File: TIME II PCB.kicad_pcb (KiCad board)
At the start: 2 copper layers, 89.9 x 62.7 mm, 116 parts, among them J1 USB_C_Receptacle, J2 SD_Card, J21 Conn_01x02_Male, J3 Conn_01x02_Male, J4 Conn_01x06_Pin, J5 Conn_01x06_Pin, J6 Conn_01x06_Pin, J7 Conn_01x06_Pin, J8 Conn_01x06_Pin, Q1 VNP10N07, Q2 VNP10N07, Q3 VNP10N07, Q4 VNP10N07, Q5 VNP10N07, Q6 NMOS, Q7 PMOS, SW1 PTS647SM38SMTR2LFS, SW2 PTS647SM38SMTR2LFS, SW3 SW_SPDT, SW4 SW_SPDT, SW5 SW_SPDT, SW6 SW_SPDT, SW7 SW_SPDT, U1 ESP32-S2-SOLO, U2 ADP2303, U3 LTC4420CMSE-PBF

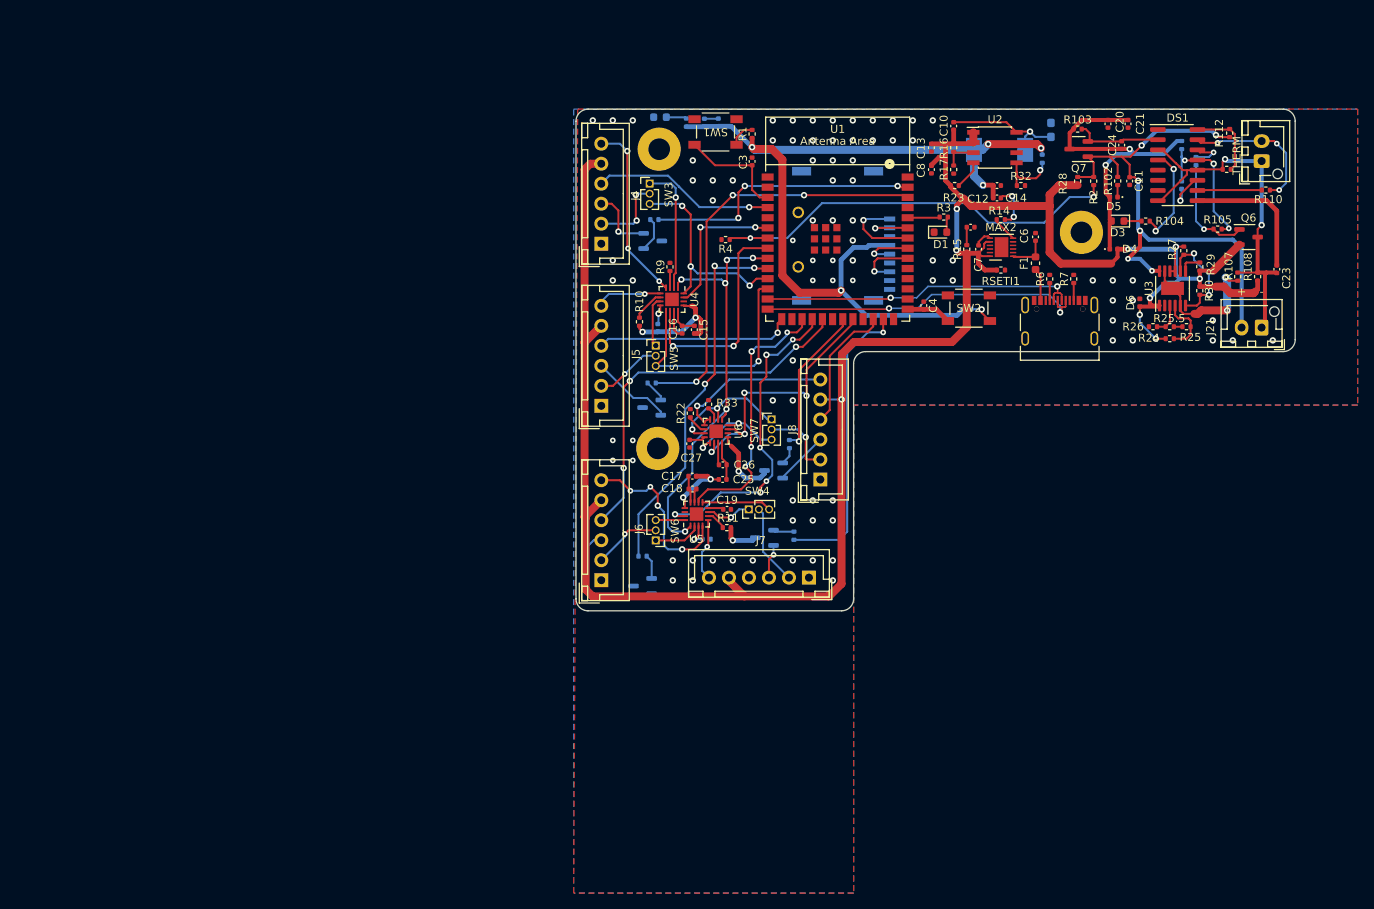
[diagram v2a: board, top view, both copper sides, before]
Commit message: new board
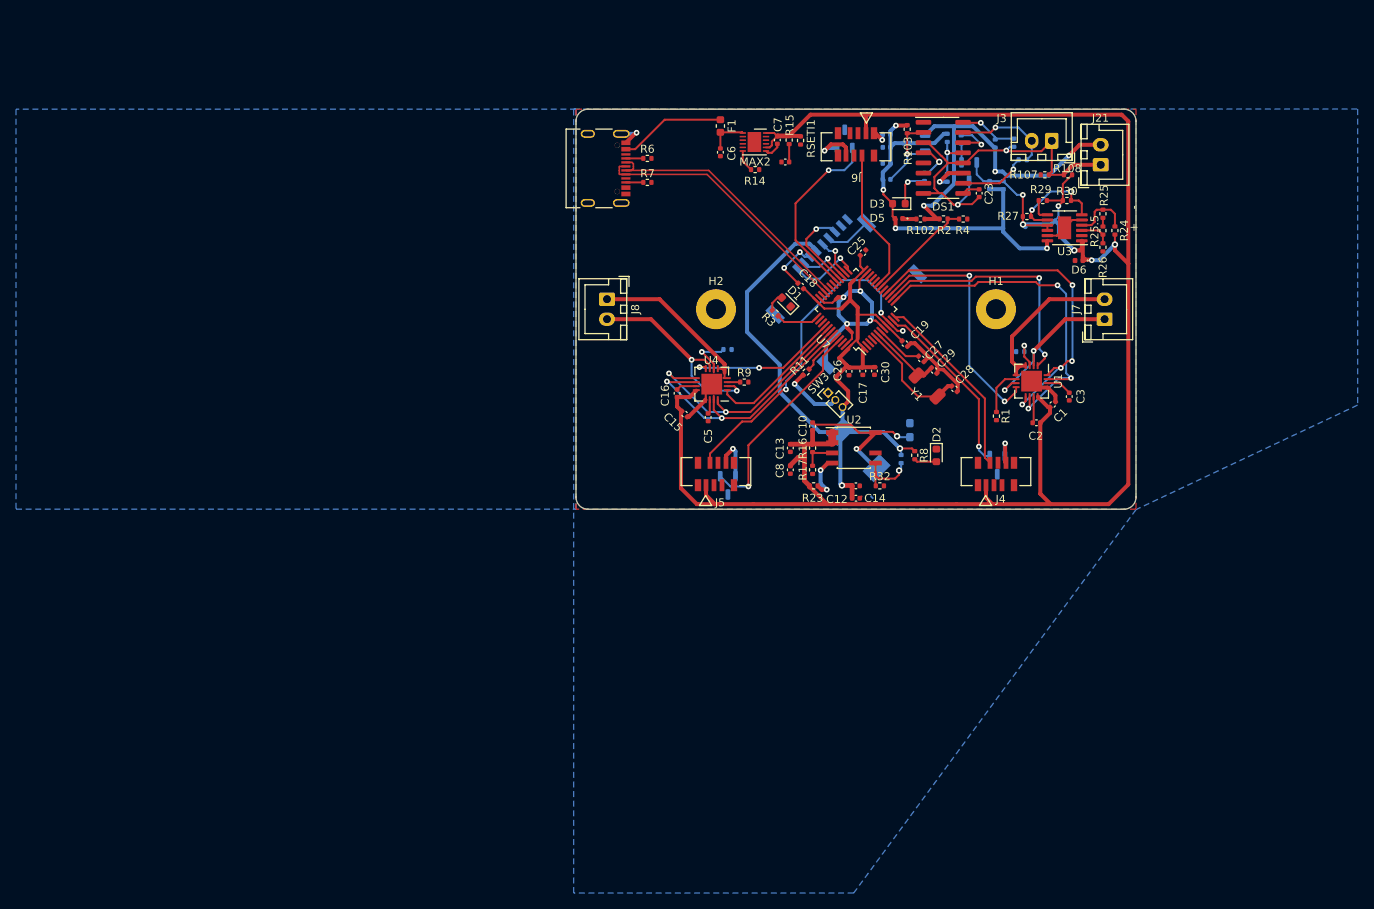
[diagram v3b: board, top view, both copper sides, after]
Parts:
- removed ? (x2): , 
- removed C4: .1uF, Capacitor_SMD:C_0402_1005Metric
- removed Q2, Q3: VNP10N07, Package_TO_SOT_SMD:SOT-23-3
- removed R105: R, Resistor_SMD:R_0402_1005Metric
- removed R13, R18, R19, R21, R5: 1.5k, Resistor_SMD:R_0402_1005Metric
- removed R20: 10k, Resistor_SMD:R_0402_1005Metric
- removed R22, R33: .33, Resistor_SMD:R_0402_1005Metric
- removed REF**: MountingHole_2.7mm_M2.5_Pad, MountingHole:MountingHole_2.7mm_M2.5_Pad
- removed SW1, SW2: PTS647SM38SMTR2LFS, button:SW_PTS647SM38SMTR2LFS_CNK
- removed SW4, SW5, SW6, SW7: SW_SPDT, Connector_PinHeader_1.27mm:PinHeader_1x03_P1.27mm_Vertical
- removed U5, U6: ~, Package_DFN_QFN:QFN-16-1EP_3x3mm_P0.5mm_EP1.7x1.7mm
- added C28: 26pF, Capacitor_SMD:C_0402_1005Metric, F.Cu at (187.7, 98.6)
- added C29: 26pF, Capacitor_SMD:C_0402_1005Metric, F.Cu at (185.2, 96.3)
- added C30: 100nF, Capacitor_SMD:C_0402_1005Metric, F.Cu at (177.7, 96.3)
- added H1: MountingHole_Pad, MountingHole:MountingHole_2.5mm_Pad, F.Cu at (192.9, 88.6)
- added H2: MountingHole_Pad, MountingHole:MountingHole_2.5mm_Pad, F.Cu at (157.9, 88.6)
- added U7: STM32F103C8Tx, Package_QFP:LQFP-48_7x7mm_P0.5mm, F.Cu at (175.4, 88.6)
- added Y1: 16 khz, crystal:abm3, F.Cu at (184.3, 98.2)
- C1: value 1uF -> 10uF; moved to F.Cu
- C11, C20, C21, C24, D4, Q6, Q7, R10, R104, R110, R112, R113, R28: moved to B.Cu
- C17, C25: value 10uF -> 100nF
- C18: value 0.01uF -> 100nF
- C19, C27: value 2.2pF -> 100nF
- C2: value .1uF -> 0.01uF; moved to F.Cu
- C26: value 0.01uF -> 10uF
- C3: value .1uF -> 2.2pF
- C5, D2, R8: moved to F.Cu
- J21, J3: footprint Connector_JST:JST_XH_B2B-XH-AM_1x02_P2.50mm_Vertical -> Connector_JST:JST_XH_B2B-XH-A_1x02_P2.50mm_Vertical
- J4, J5, J6: value Conn_01x06_Pin -> Conn_01x06; footprint Connectors_JST:JST_XH_B06B-XH-A_06x2.50mm_Straight -> ffc_conn:CON_525590652_MOL
- J7, J8: value Conn_01x06_Pin -> Conn_01x02_Male; footprint Connectors_JST:JST_XH_B06B-XH-A_06x2.50mm_Straight -> Connector_JST:JST_XH_B2B-XH-A_1x02_P2.50mm_Vertical
- R1: value 10k -> .33
- R11: value .33 -> 10k
- U1: value ESP32-S2-SOLO -> ~; footprint Espressif:ESP32-S2-SOLO -> Package_DFN_QFN:WQFN-16-1EP_4x4mm_P0.5mm_EP2.6x2.6mm
- U4: footprint Package_DFN_QFN:QFN-16-1EP_3x3mm_P0.5mm_EP1.7x1.7mm -> Package_DFN_QFN:WQFN-16-1EP_4x4mm_P0.5mm_EP2.6x2.6mm
- moved J6 63.1 mm to (175.4, 68.0), turned to 180 degrees
- moved Q5 61.3 mm to (174.0, 67.3), turned to 90 degrees
- moved J1 61.1 mm to (143.2, 71.0), turned to -90 degrees
- moved J4 57.1 mm to (192.9, 109.2), turned to 0 degrees
- moved C2 56.0 mm to (198.0, 102.8), turned to 180 degrees
- moved C1 54.7 mm to (200.0, 100.5), turned to 45 degrees
- moved R7 54.6 mm to (149.3, 72.7), turned to 0 degrees
- moved D2 54.6 mm to (185.4, 106.9), turned to -90 degrees
- moved R6 52.5 mm to (149.3, 69.8), turned to 0 degrees
- moved Q4 51.4 mm to (193.1, 108.1), turned to -90 degrees
- moved R8 50.4 mm to (182.7, 106.9), turned to -90 degrees
- moved C3 49.4 mm to (202.1, 99.5)
- moved J7 49.1 mm to (206.5, 89.8), turned to 90 degrees
- moved R1 46.6 mm to (193.0, 102.0), turned to -90 degrees
- moved R12 45.7 mm to (195.9, 93.9), turned to 180 degrees
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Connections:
- C1 pad 1: 3v3 -> 5v
- C15 pad 1: Net-(U4-VM) -> 5v
- C16 pad 1: Net-(U4-VM) -> 5v
- C17 pad 1: Net-(U5-VM) -> 3v3
- C18 pad 1: Net-(U5-VM) -> 3v3
- C18 pad 2: Net-(U5-VCP) -> GND
- C19 pad 1: Net-(U5-NFAULT) -> 3v3
- C2 pad 1: 3v3 -> 5v
- C2 pad 2: GND -> Net-(U1-VCP)
- C20 pad 1: LOAD -> BAT
- C21 pad 1: LOAD -> BAT
- C24 pad 1: LOAD -> BAT
- C25 pad 1: Net-(U6-VM) -> 3v3
- C26 pad 1: Net-(U6-VM) -> 3v3
- C26 pad 2: Net-(U6-VCP) -> GND
- C27 pad 1: Net-(U6-NFAULT) -> /nrst
- C3 pad 1: GND -> Net-(U1-VINT)
- C3 pad 2: Net-(U1-EN) -> GND
- C5 pad 1: Net-(U4-NFAULT) -> Net-(U4-VINT)
- D3 pad 2: LOAD -> BAT
- D4 pad 1: LOAD -> BAT
- D5 pad 2: LOAD -> BAT
- J21 pad 2: BAT -> BAT_REAL
- J4 pad 1: GND -> 5v
- J4 pad 2: ACTUATOR_1 -> therm_1
- J4 pad 3: Net-(J4-Pin_3) -> unconnected-(J4-Pin_3-Pad3)
- J4 pad 4: therm_1 -> GND
- J4 pad 5: 5v -> unconnected-(J4-Pin_5-Pad5)
- J4 pad 6: MOTOR_1A -> Net-(J4-Pin_6)
- J5 pad 1: GND -> 5v
- J5 pad 2: ACTUATOR_2 -> therm_2
- J5 pad 3: Net-(J5-Pin_3) -> unconnected-(J5-Pin_3-Pad3)
- J5 pad 4: therm_2 -> GND
- J5 pad 5: 5v -> unconnected-(J5-Pin_5-Pad5)
- J5 pad 6: MOTOR_2A -> Net-(J5-Pin_6)
- J6 pad 1: GND -> 5v
- J6 pad 2: ACTUATOR_3 -> therm_3
- J6 pad 3: Net-(J6-Pin_3) -> unconnected-(J6-Pin_3-Pad3)
- J6 pad 4: therm_3 -> GND
- J6 pad 5: 5v -> unconnected-(J6-Pin_5-Pad5)
- J6 pad 6: MOTOR_3A -> Net-(J6-Pin_6)
- J7 pad 1: GND -> MOTOR_2
- J7 pad 2: ACTUATOR_4 -> MOTOR_2A
- J8 pad 1: GND -> MOTOR_1A
- J8 pad 2: ACTUATOR_5 -> MOTOR_1
- Q1 pad 1: Net-(Q1-G) -> heater_2
- Q1 pad 2: Net-(J5-Pin_3) -> Net-(J5-Pin_6)
- Q4 pad 1: Net-(Q4-G) -> heater_1
- Q4 pad 2: Net-(J4-Pin_3) -> Net-(J4-Pin_6)
- Q5 pad 1: Net-(Q5-G) -> heater_3
- Q5 pad 2: Net-(J6-Pin_3) -> Net-(J6-Pin_6)
- Q7 pad 1: BAT -> BAT_REAL
- Q7 pad 3: LOAD -> BAT
- R1 pad 1: 3v3 -> Net-(U1-BISEN)
- R1 pad 2: Net-(R1-Pad2) -> GND
- R101 pad 1: LOAD -> BAT
- R102 pad 2: BAT -> BAT_REAL
- R103 pad 1: LOAD -> BAT
- R11 pad 1: Net-(U5-BISEN) -> Net-(SW3-B)
- R11 pad 2: GND -> Net-(U7-BOOT0)
- R112 pad 1: BAT -> BAT_REAL
- R12 pad 1: Net-(U5-AISEN) -> Net-(U1-AISEN)
- R2 pad 1: BAT -> BAT_REAL
- SW3 pad 1: MOTOR_1 -> GND
- SW3 pad 2: ACTUATOR_1 -> Net-(SW3-B)
- SW3 pad 3: SERVO_1 -> 3v3
- U1 pad 1: GND -> MOT_CON2
- U1 pad 10: heater_3 -> SERVO_2A
- U1 pad 11: SERVO_1 -> Net-(U1-VCP)
- U1 pad 12: SERVO_2 -> 5v
- U1 pad 13: D- -> GND
- U1 pad 14: D+ -> Net-(U1-VINT)
- U1 pad 15: therm_2 -> SERVO_2A
- U1 pad 16: unconnected-(U1-GPIO46-Pad16) -> SERVO_2
- U1 pad 17: SERVO_4A -> GND
- U1 pad 2: unconnected-(U1-3V3-Pad2) -> MOTOR_2
- U1 pad 3: Net-(U1-EN) -> Net-(U1-AISEN)
- U1 pad 4: therm_1 -> MOTOR_2A
- U1 pad 5: unconnected-(U1-GPIO5/TOUCH5/ADC1_CH4-Pad5) -> MOTOR_2A
- U1 pad 6: SERVO_1A -> Net-(U1-BISEN)
- U1 pad 7: V_MON -> MOTOR_2
- U1 pad 8: SERVO_2A -> MOT_MON_2
- U1 pad 9: MOT_CON -> SERVO_2
- U4 pad 1: MOT_CON -> MOT_CON1
- U4 pad 10: SERVO_2A -> SERVO_1A
- U4 pad 12: Net-(U4-VM) -> 5v
- U4 pad 14: MOT_MON_1 -> Net-(U4-VINT)
- U4 pad 17: (no net) -> GND
- U4 pad 5: MOTOR_2A -> MOTOR_1A
- U4 pad 7: MOTOR_2 -> MOTOR_1
- U4 pad 8: Net-(U4-NFAULT) -> MOT_MON_1
- U4 pad 9: SERVO_2 -> SERVO_1
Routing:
- net MOT_CON: track 53.3 -> 0.00 mm, vias 6 -> 0
- net BAT_REAL: track 0.00 -> 45.0 mm, vias 0 -> 3
- net SERVO_3A: track 40.1 -> 0.00 mm, vias 6 -> 0
- net LOAD: track 40.0 -> 0.00 mm, vias 2 -> 0
- net V_MON: track 53.4 -> 13.6 mm, vias 2 -> 0
- net heater_4: track 36.6 -> 0.00 mm, vias 1 -> 0
- net SERVO_4A: track 33.4 -> 0.00 mm, vias 4 -> 0
- net SERVO_5A: track 33.2 -> 0.00 mm, vias 4 -> 0
- net MOT_CON2: track 0.00 -> 31.2 mm, vias 0 -> 2
- net MOT_MON_2: track 0.00 -> 31.1 mm, vias 0 -> 2
- net therm_3: track 46.7 -> 18.1 mm, vias 3 -> 0
- net heater_2: track 51.9 -> 27.1 mm, vias 3 -> 1
- net heater_3: track 47.0 -> 22.9 mm, vias 3 -> 1
- net MOTOR_3A: track 22.3 -> 0.00 mm, vias 4 -> 0
- net 5v: track 280.4 -> 258.8 mm, vias 9 -> 6
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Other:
- board size 89.9 x 62.7 mm -> 70 x 50 mm
- board text removed: "THERM"
